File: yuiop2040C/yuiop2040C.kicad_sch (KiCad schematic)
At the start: 31 parts, among them J1 Conn_01x20, J2 Conn_01x20, J3 Conn_01x03, U1 RP2040, U2 W25Q16JVSS, U3 MIC5219-3.3YM5, Y1 FA238V 12.000000MHz 10.0 +50.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

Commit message: YUIOP2040C: start plotting
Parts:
- U1: footprint RP2040_minimal:RP2040-QFN-56-r2 -> RP2040_minimal:RP2040-QFN-56
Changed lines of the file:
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@@
       (effects (font (size 1.27 1.27)) (justify left))
     )
-    (property "Footprint" "RP2040_minimal:RP2040-QFN-56-r2" (id 2) (at 104.14 130.81 0)
+    (property "Footprint" "RP2040_minimal:RP2040-QFN-56" (id 2) (at 104.14 130.81 0)
       (effects (font (size 1.27 1.27)) hide)
     )
@@
     )
     (path "/0c64a8a2-476d-4ce5-9a4f-cce66f41d837"
-      (reference "U1") (unit 1) (value "RP2040") (footprint "RP2040_minimal:RP2040-QFN-56-r2")
+      (reference "U1") (unit 1) (value "RP2040") (footprint "RP2040_minimal:RP2040-QFN-56")
     )
     (path "/565082b3-06ce-46fa-857c-fecdf53c89f1"

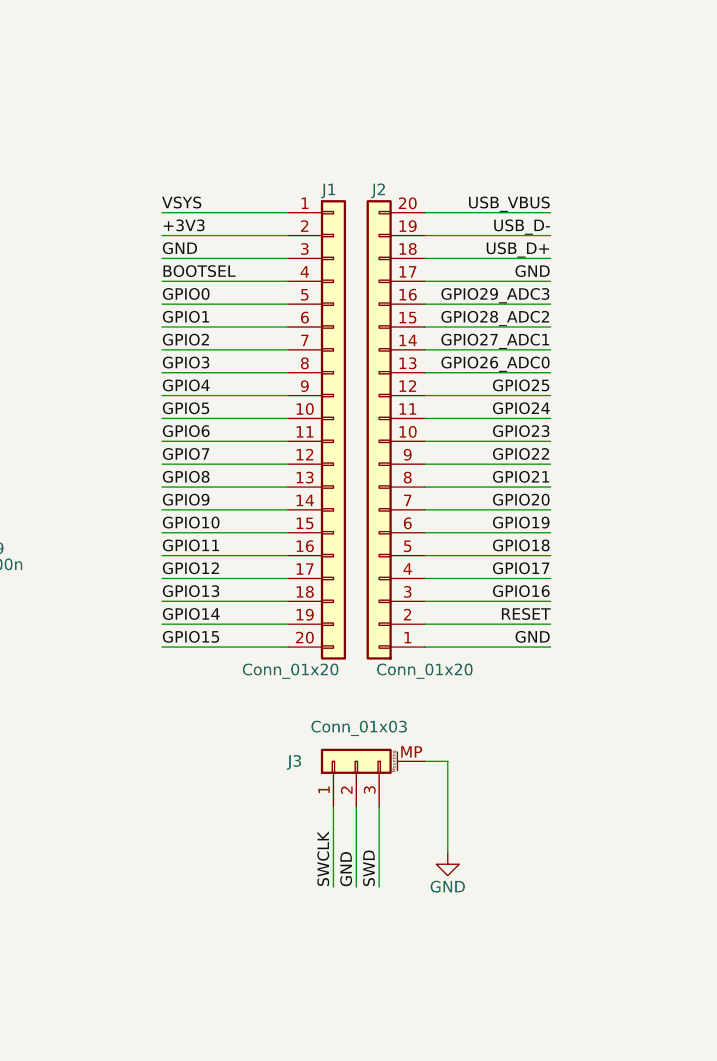
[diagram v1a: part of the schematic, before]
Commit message: fix
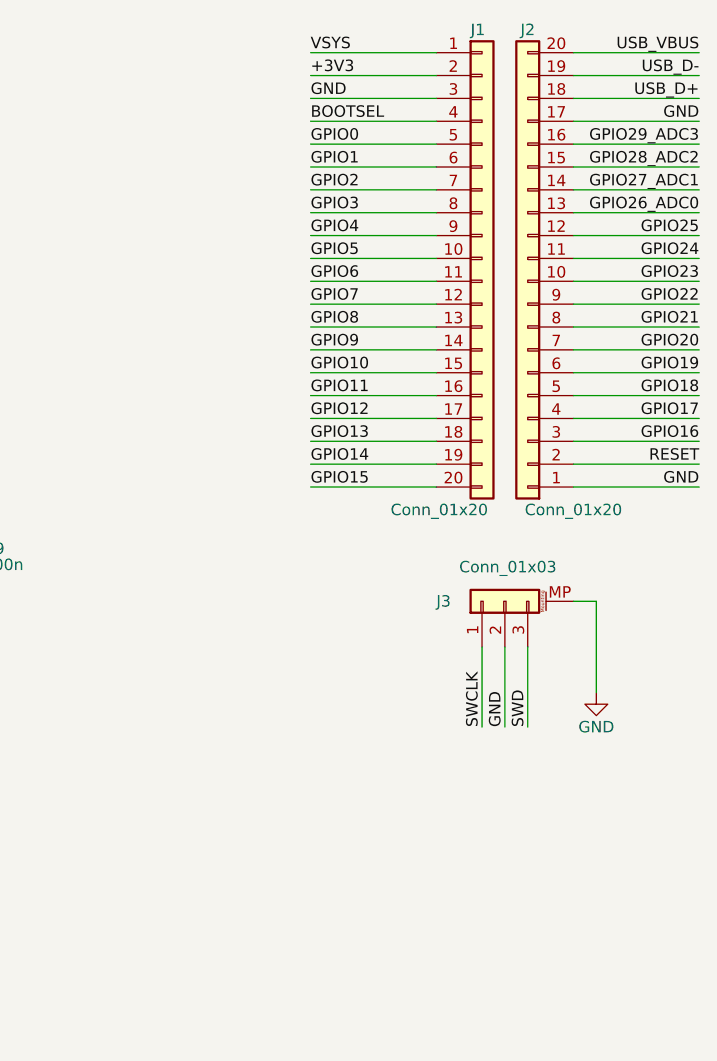
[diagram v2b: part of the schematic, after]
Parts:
- C1, C12, C13, C14, C2, C3, C4, C5, C6, C7, C8, C9: footprint Capacitor_SMD:C_0603_1608Metric -> Capacitor_SMD:C_0402_1005Metric
- R1, R2, R3, R4, R5, R6: footprint Resistor_SMD:R_0603_1608Metric -> Resistor_SMD:R_0402_1005Metric
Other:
- moved on the sheet: J1, J2, J3
